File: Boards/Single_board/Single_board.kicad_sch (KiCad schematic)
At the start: 8 parts, among them J1 Conn_01x04_Socket, J2 Conn_01x04_Socket, Q1 SI2306

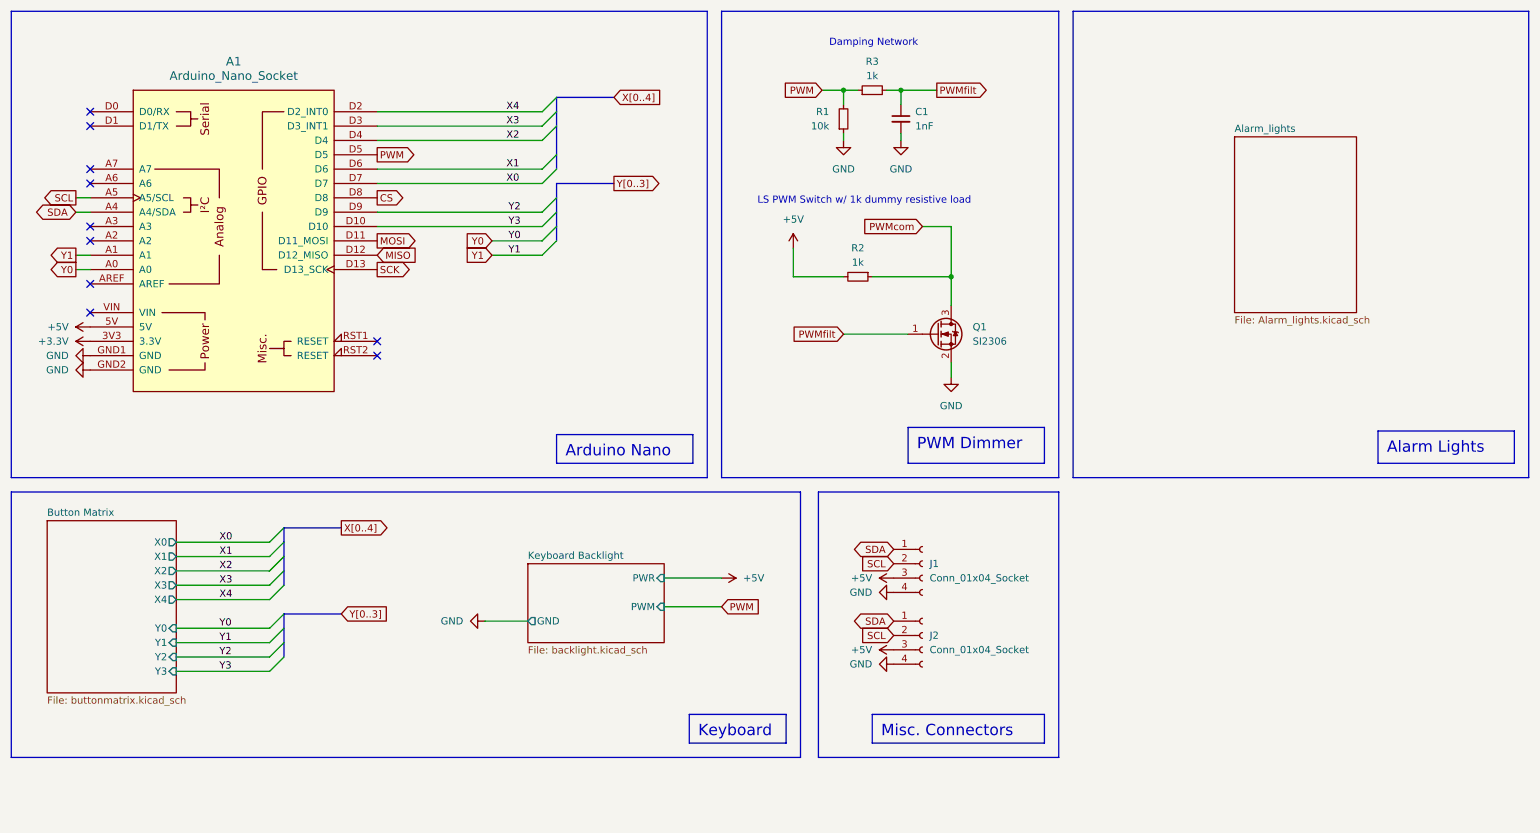
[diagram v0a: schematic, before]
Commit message: some progress on the arduino boilerplate
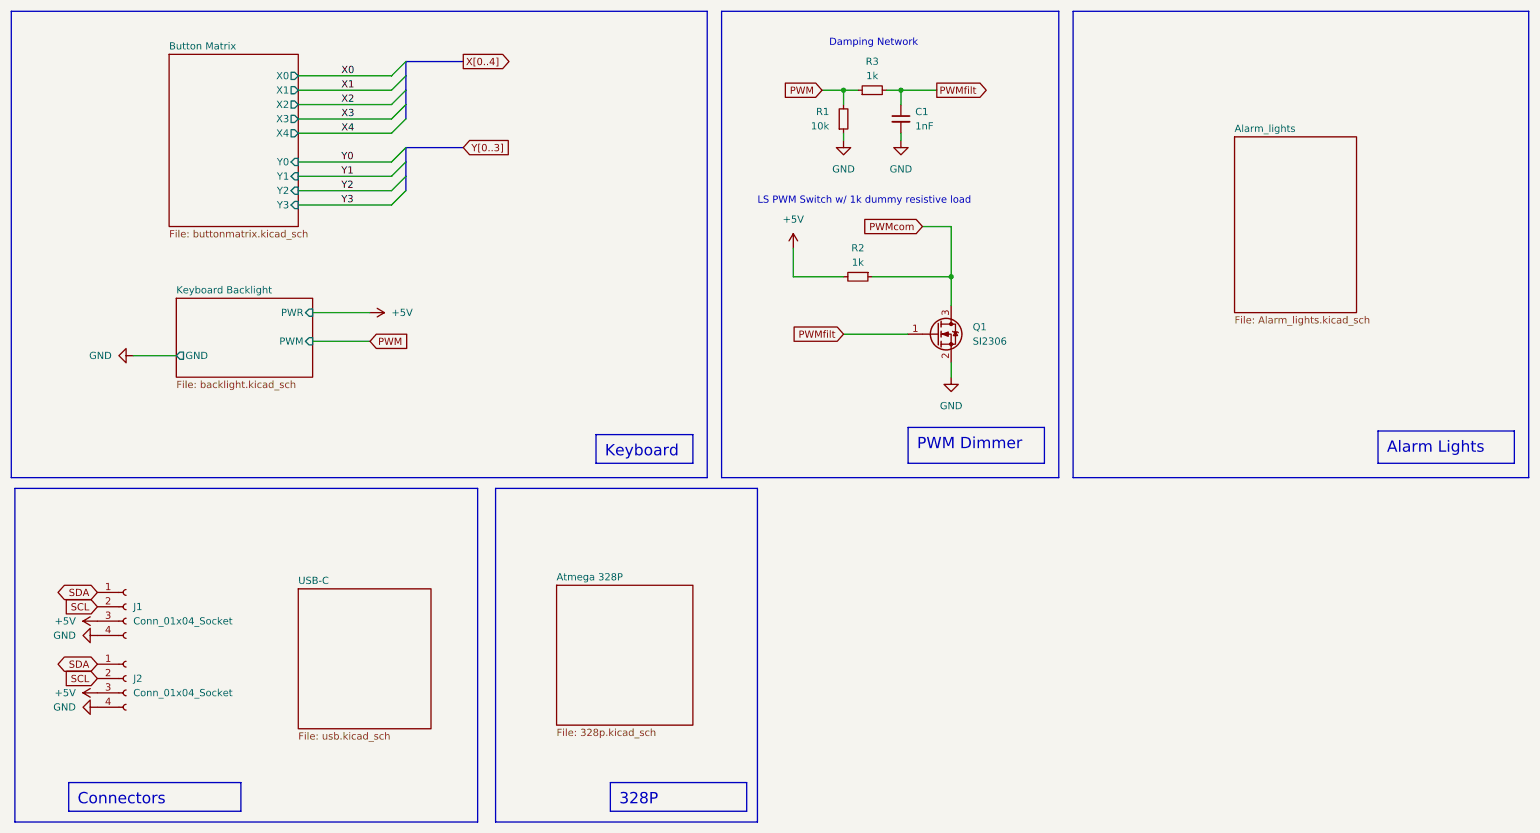
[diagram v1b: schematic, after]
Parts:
- removed A1: Arduino_Nano_Socket, PCM_arduino-library:Arduino_Nano_Socket, symbol PCM_arduino-library:Arduino_Nano_Socket
- C1: footprint Capacitor_SMD:C_1206_3216Metric_Pad1.33x1.80mm_HandSolder -> Capacitor_SMD:C_0805_2012Metric
- Q1: footprint Package_TO_SOT_SMD:SOT-23-3 -> Package_TO_SOT_SMD:SOT-23
- R1, R2, R3: footprint Resistor_SMD:R_1206_3216Metric_Pad1.30x1.75mm_HandSolder -> Resistor_SMD:R_1206_3216Metric
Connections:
- no-connect marks 10 -> 0
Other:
- added sheet Atmega 328P (328p.kicad_sch)
- added sheet USB-C (usb.kicad_sch)
- title: DSKY Main Board -> DSKY Board
- moved on the sheet: J1, J2
